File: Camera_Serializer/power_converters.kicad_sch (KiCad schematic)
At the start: 9 parts, among them U3 TPS62133RGTR

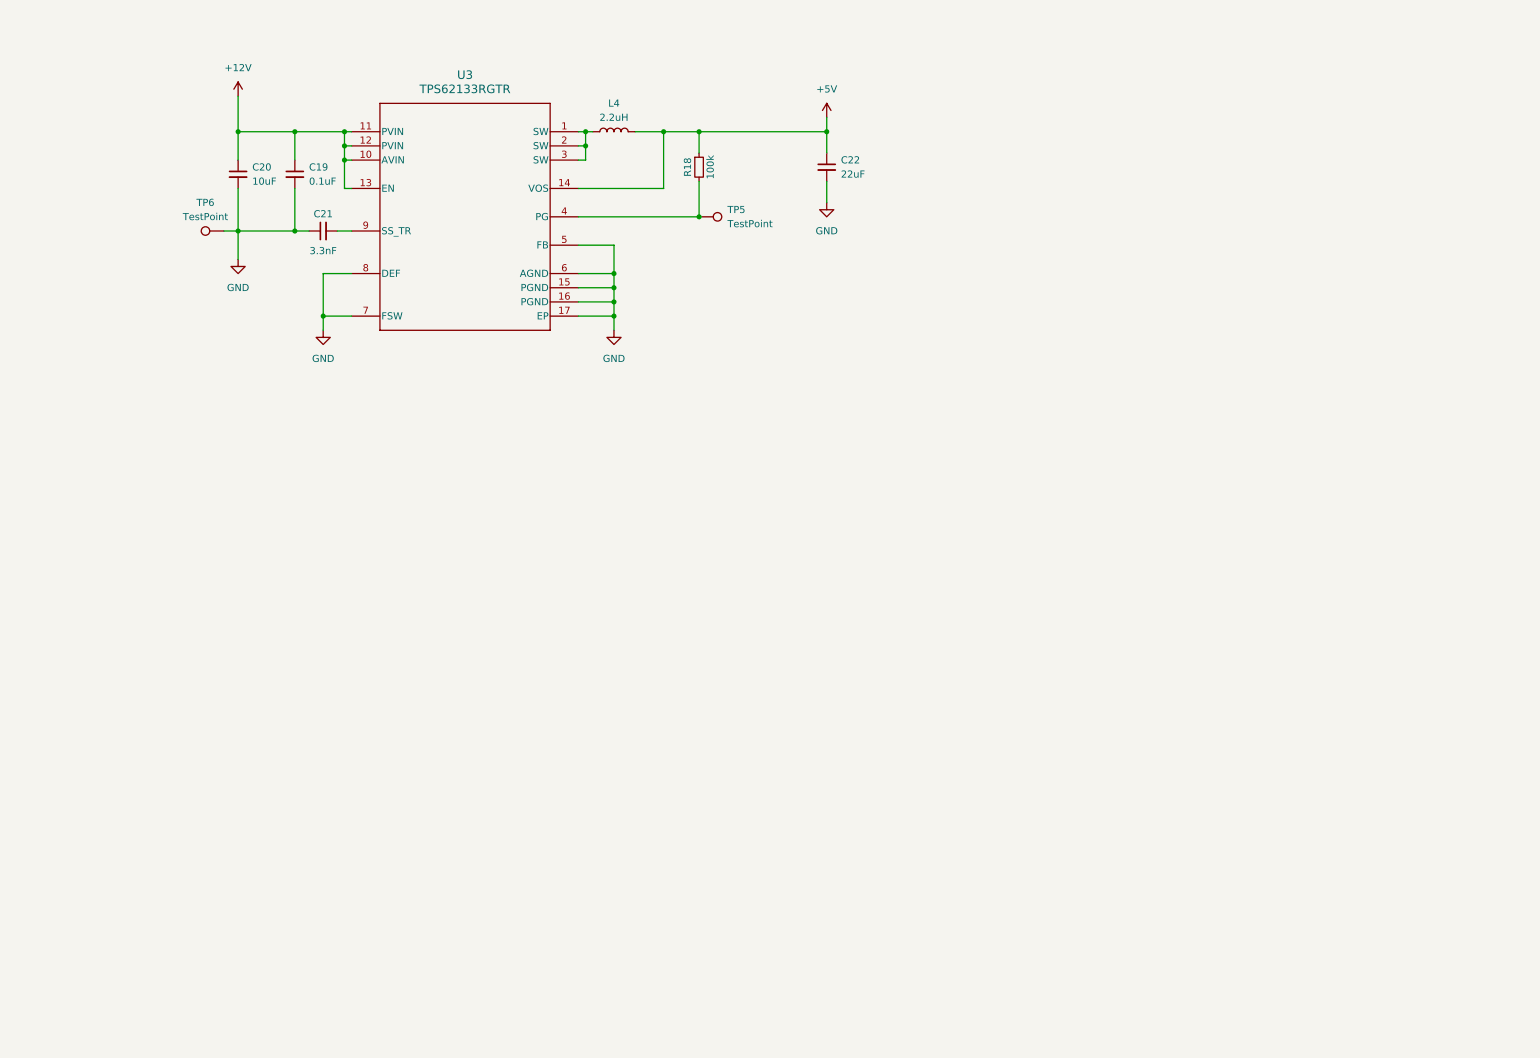
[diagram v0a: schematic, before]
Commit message: Finished power converters
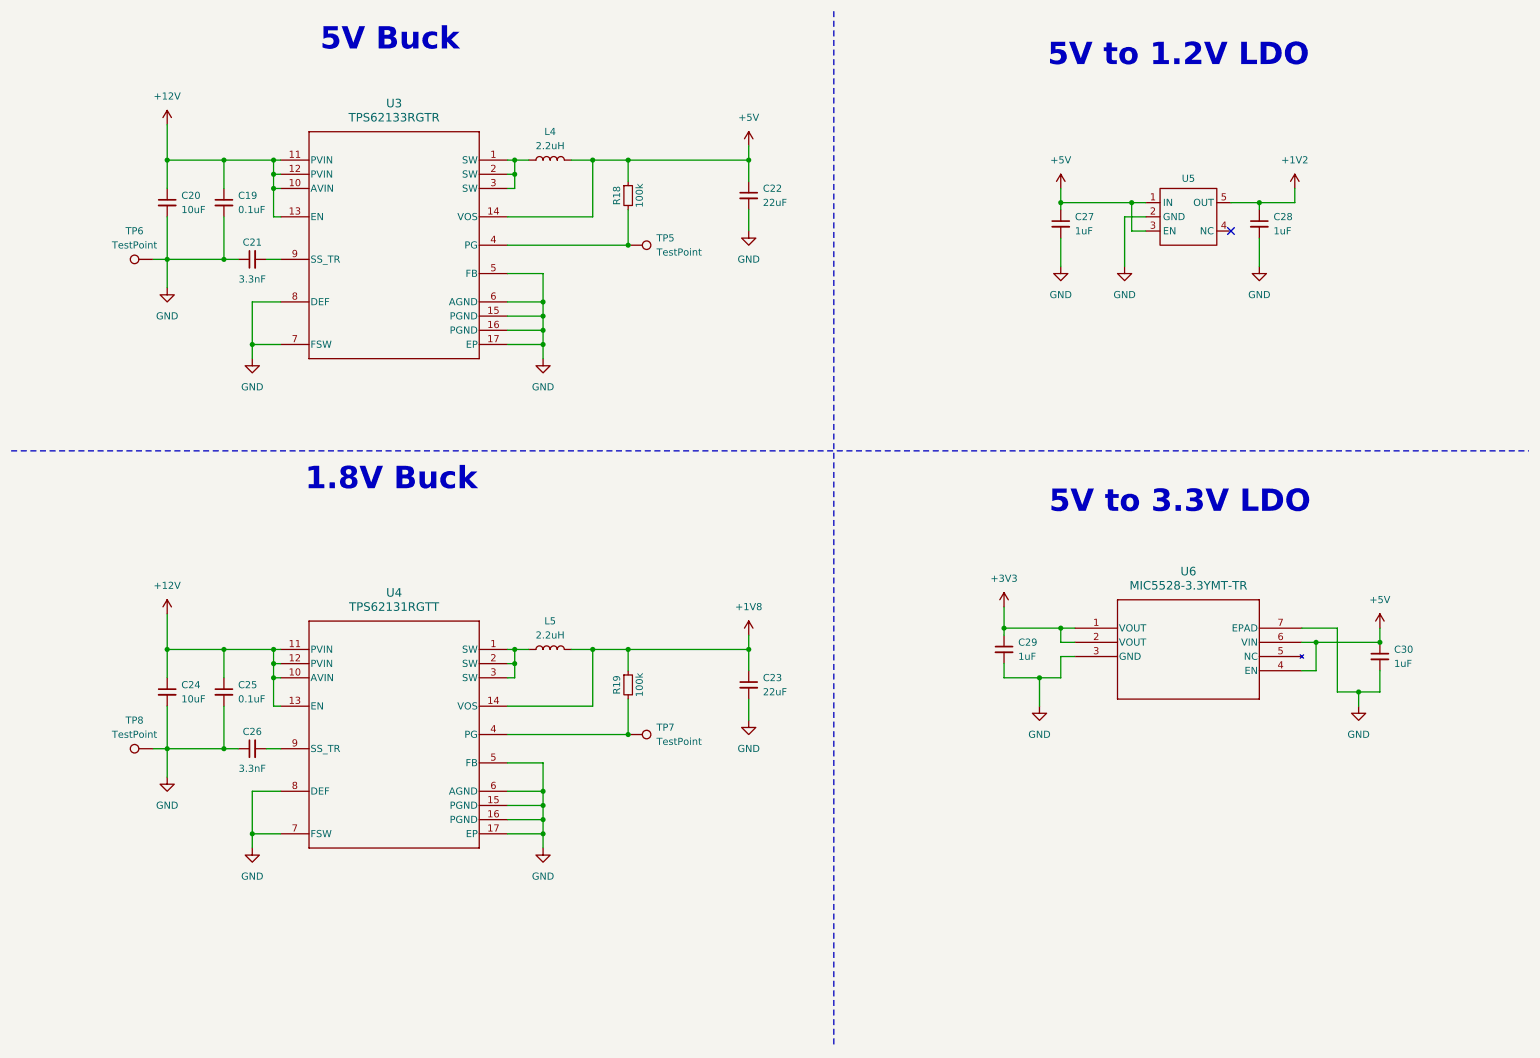
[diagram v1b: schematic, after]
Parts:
- added C23: 22uF, Capacitor_SMD:C_0603_1608Metric_Pad1.08x0.95mm_HandSolder, symbol Device:C_Small
- added C24: 10uF, Capacitor_SMD:C_0805_2012Metric_Pad1.18x1.45mm_HandSolder, symbol Device:C_Small
- added C25: 0.1uF, Capacitor_SMD:C_0402_1005Metric_Pad0.74x0.62mm_HandSolder, symbol Device:C_Small
- added C26: 3.3nF, Capacitor_SMD:C_0402_1005Metric_Pad0.74x0.62mm_HandSolder, symbol Device:C_Small
- added C27, C28, C29, C30: 1uF, symbol Device:C_Small
- added L5: 2.2uH, CameraServer_Footprints:IFSC1515AHER2R2M01, symbol Device:L
- added R19: 100k, Resistor_SMD:R_0402_1005Metric_Pad0.72x0.64mm_HandSolder, symbol Device:R_Small
- added TP7, TP8: TestPoint, TestPoint:TestPoint_Pad_D2.0mm, symbol Connector:TestPoint
- added U4: TPS62131RGTT, Snapeda:RGT0016C, symbol Snapeda:TPS62131RGTT
- added U5: ~, CameraServer_Footprints:NCP114ASN120T1G, symbol CameraServer_Symbols:NCP114ASN120T1G
- added U6: MIC5528-3.3YMT-TR, Snapeda:TDFN6_1P2X1P2_MCH, symbol Snapeda:MIC5528-3.3YMT-TR
- C22: footprint (none) -> Capacitor_SMD:C_0603_1608Metric_Pad1.08x0.95mm_HandSolder
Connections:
- net +12V: now also C24.1, C25.1, U4.10 (AVIN), U4.11 (PVIN), U4.12 (PVIN), U4.13 (EN)
- net +5V: now also C27.1, C30.1, U5.1 (IN), U5.3 (EN), U6.4 (EN), U6.6 (VIN)
- net GND: now also C23.2, C24.2, C25.2, C26.1, C27.2, C28.2, C29.2, C30.2, TP8.1, U4.15 (PGND), U4.16 (PGND), U4.17 (EP), U4.5 (FB), U4.6 (AGND), U4.7 (FSW), U4.8 (DEF), U5.2 (GND), U6.3 (GND), U6.7 (EPAD)
- new net: L5.1, U4.1 (SW), U4.2 (SW), U4.3 (SW)
- new net: R19.2, TP7.1, U4.4 (PG)
- new net: C26.2, U4.9 (SS_TR)
- new net +1V2: C28.1, U5.5 (OUT)
- new net +1V8: C23.1, L5.2, R19.1, U4.14 (VOS)
- new net +3V3: C29.1, U6.1 (VOUT), U6.2 (VOUT)
- no-connect marks 0 -> 1
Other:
- note added: "1.8V Buck"
- note added: "5V Buck"
- note added: "5V to 1.2V LDO"
- note added: "5V to 3.3V LDO"
- moved on the sheet: C19, C20, C21, C22, L4, R18, TP5, TP6, U3

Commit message: Finishe schematic
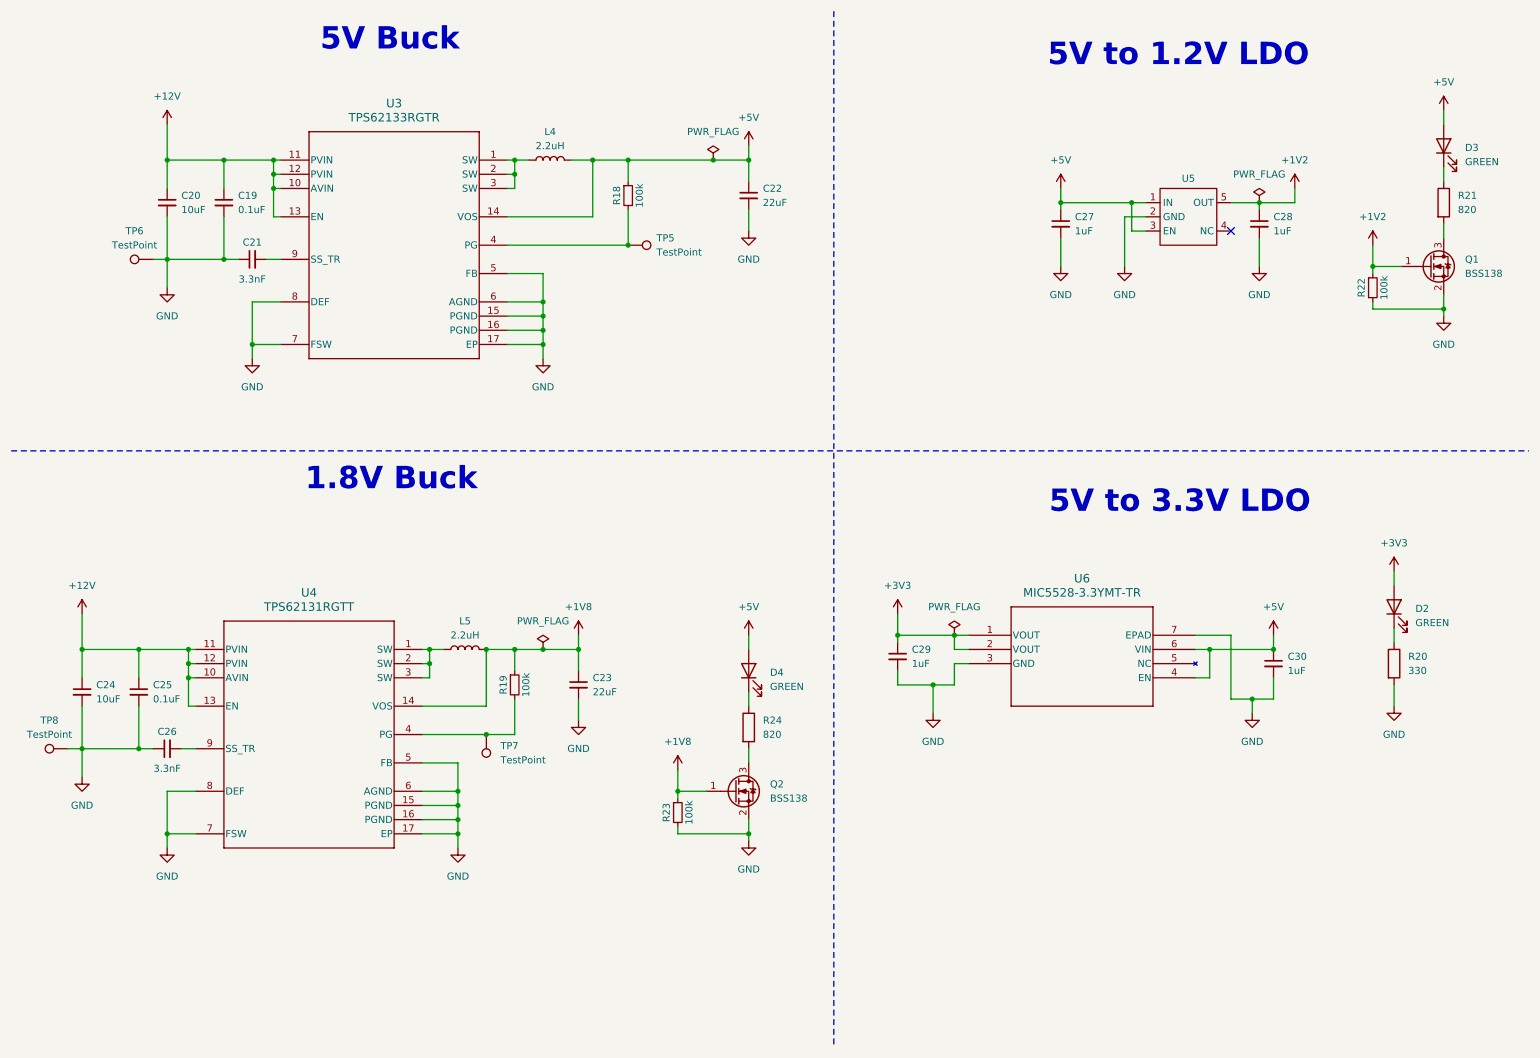
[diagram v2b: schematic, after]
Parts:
- added D2, D3, D4: GREEN, LED_SMD:LED_0603_1608Metric_Pad1.05x0.95mm_HandSolder, symbol Device:LED
- added Q1, Q2: BSS138, Package_TO_SOT_SMD:SOT-23, symbol Transistor_FET:BSS138
- added R20: 330, Resistor_SMD:R_0603_1608Metric_Pad0.98x0.95mm_HandSolder, symbol Device:R
- added R21, R24: 820, Resistor_SMD:R_0603_1608Metric_Pad0.98x0.95mm_HandSolder, symbol Device:R
- added R22, R23: 100k, Resistor_SMD:R_0402_1005Metric_Pad0.72x0.64mm_HandSolder, symbol Device:R_Small
- C27, C28, C29, C30: footprint (none) -> Capacitor_SMD:C_0402_1005Metric_Pad0.74x0.62mm_HandSolder
- TP5, TP6, TP7, TP8: footprint TestPoint:TestPoint_Pad_D2.0mm -> TestPoint:TestPoint_Pad_D1.0mm
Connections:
- net +1V2: now also Q1.1 (G), R22.1
- net +1V8: now also Q2.1 (G), R23.1
- net +3V3: now also D2.2 (A)
- net +5V: now also D3.2 (A), D4.2 (A)
- net GND: now also Q1.2 (S), Q2.2 (S), R20.2, R22.2, R23.2
- new net: D2.1 (K), R20.1
- new net: D4.1 (K), R24.1
- new net: Q2.3 (D), R24.2
- new net: D3.1 (K), R21.1
- new net: Q1.3 (D), R21.2
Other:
- moved on the sheet: C23, C24, C25, C26, C29, C30, L5, R19, TP7, TP8, U4, U6

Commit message: Layout started
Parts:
- U4: footprint Snapeda:RGT0016C -> CameraServer_Footprints:TPS62133RGTR
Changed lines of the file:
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@@
 			)
 		)
-		(property "Footprint" "Snapeda:RGT0016C"
+		(property "Footprint" "CameraServer_Footprints:TPS62133RGTR"
 			(at 66.04 142.24 0)
 			(effects
